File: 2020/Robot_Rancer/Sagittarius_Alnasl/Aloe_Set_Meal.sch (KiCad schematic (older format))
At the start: 235 parts, among them J1 SWD, J10 MOTOR1, J11 MOTOR3, J12 MOTOR5, J13 BATT_IN, J14 3522-2, J15 microSD, J16 SERIAL1, J17 VOLTMETER, J18 TO_VOLTMETER, J2 ADC, J3 ADC_Vdd, J4 SERIAL0, J5 ENC, J6 MOTOR0, J7 MOTOR2, J8 MOTOR4, J9 SERVO, Q1 NVMFD5C446NLT1G, Q10 NVMFD5C446NLT1G, Q11 NVMFD5C446NLT1G, Q12 NVMFD5C446NLT1G, Q13 FET_P, Q14 FET_N, Q15 FET_P, Q16 NPN, Q2 NVMFD5C446NLT1G, Q3 NVMFD5C446NLT1G, Q4 NVMFD5C446NLT1G, Q5 NVMFD5C446NLT1G, Q6 NVMFD5C446NLT1G, Q7 NVMFD5C446NLT1G, Q8 NVMFD5C446NLT1G, Q9 NVMFD5C446NLT1G, SW1 RST, SW2 SW0, SW3 SW1, SW4 EMG, SW5 MAIN_SW, U1 BD9G101G, U10 NCP5104, U11 NCP5104, U12 NCP5104, U13 NCP5104, U14 NCP5104, U15 NCP5104, U16 NCP5104, U17 NCP5104, U18 V23086-C1001, U19 LOGO, U2 MCP2221A, U20 LOGO, U21 LOGO, U22 AQM0802, U23 74HCT04, U24 74HC02, U25 74HC02, U26 74HC02, U27 LOGO, U28 FULLCOLOR, U29 LOGO, U3 STM32F446RETx, U30 LOGO, U4 ROTARY, U5 AZ1086H, U6 NCP5104, U7 NCP5104, U8 NCP5104, U9 NCP5104, Y1 8MHz

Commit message: 抵抗値入れた
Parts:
- removed Q13: FET_P, Package_TO_SOT_SMD:SOT-23W, symbol Device:Q_PMOS_GDS
- removed Q15: FET_P, Package_TO_SOT_SMD:SOT-23W, symbol Device:Q_NMOS_GSD
- added Q13, Q15: FET_P, Package_TO_SOT_SMD:SOT-23, symbol Device:Q_PMOS_GSD
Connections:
- net +5V: now also Q13.3 (D)
- net 5Vc: now also Q13.2 (S)
- net Batt: now also Q15.2 (S)
- net at D27.1 (K), U18.2: now also Q15.3 (D)
- net at R52.2, SW4.2 (B): now also Q15.1 (G)
- net at R65.2, SW5.2 (B): now also Q13.1 (G)
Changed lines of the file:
@@
 Wire Wire Line
 	20700 7950 20750 7950
-Connection ~ 20750 7550
-$Comp
-L Device:Q_PMOS_GDS Q13
-U 1 1 5EA59B7C
-P 20650 7750
-F 0 "Q13" H 20856 7796 50  0000 L CNN
-F 1 "FET_P" H 20856 7705 50  0000 L CNN
-F 2 "Package_TO_SOT_SMD:SOT-23W" H 20850 7850 50  0001 C CNN
-F 3 "~" H 20650 7750 50  0001 C CNN
-	1    20650 7750
-	1    0    0    1
-$EndComp
 Wire Wire Line
 	21625 7550 21625 7725
@@
 Wire Wire Line
 	16350 10850 16325 10850
-$Comp
-L Device:Q_NMOS_GSD Q15
-U 1 1 5EA796FC
-P 3850 1350
-F 0 "Q15" H 4025 1150 50  0000 L CNN
-F 1 "FET_P" H 4025 1225 50  0000 L CNN
-F 2 "Package_TO_SOT_SMD:SOT-23W" H 4050 1450 50  0001 C CNN
-F 3 "~" H 3850 1350 50  0001 C CNN
-	1    3850 1350
-	1    0    0    -1
-$EndComp
 Text GLabel 2875 1200 2    50   Input ~ 0
 5Vc
@@
 Wire Wire Line
 	20600 7025 20750 7025
+$Comp
+L Device:Q_PMOS_GSD Q13
+U 1 1 5E61DA1A
+P 3850 1350
+F 0 "Q13" H 4056 1396 50  0000 L CNN
+F 1 "FET_P" H 4056 1305 50  0000 L CNN
+F 2 "Package_TO_SOT_SMD:SOT-23" H 4050 1450 50  0001 C CNN
+F 3 "~" H 3850 1350 50  0001 C CNN
+	1    3850 1350
+	1    0    0    -1
+$EndComp
+$Comp
+L Device:Q_PMOS_GSD Q15
+U 1 1 5E62C9E6
+P 20650 7750
+F 0 "Q15" H 20856 7796 50  0000 L CNN
+F 1 "FET_P" H 20856 7705 50  0000 L CNN
+F 2 "Package_TO_SOT_SMD:SOT-23" H 20850 7850 50  0001 C CNN
+F 3 "~" H 20650 7750 50  0001 C CNN
+	1    20650 7750
+	1    0    0    -1
+$EndComp
+Connection ~ 20750 7550
 $EndSCHEMATC

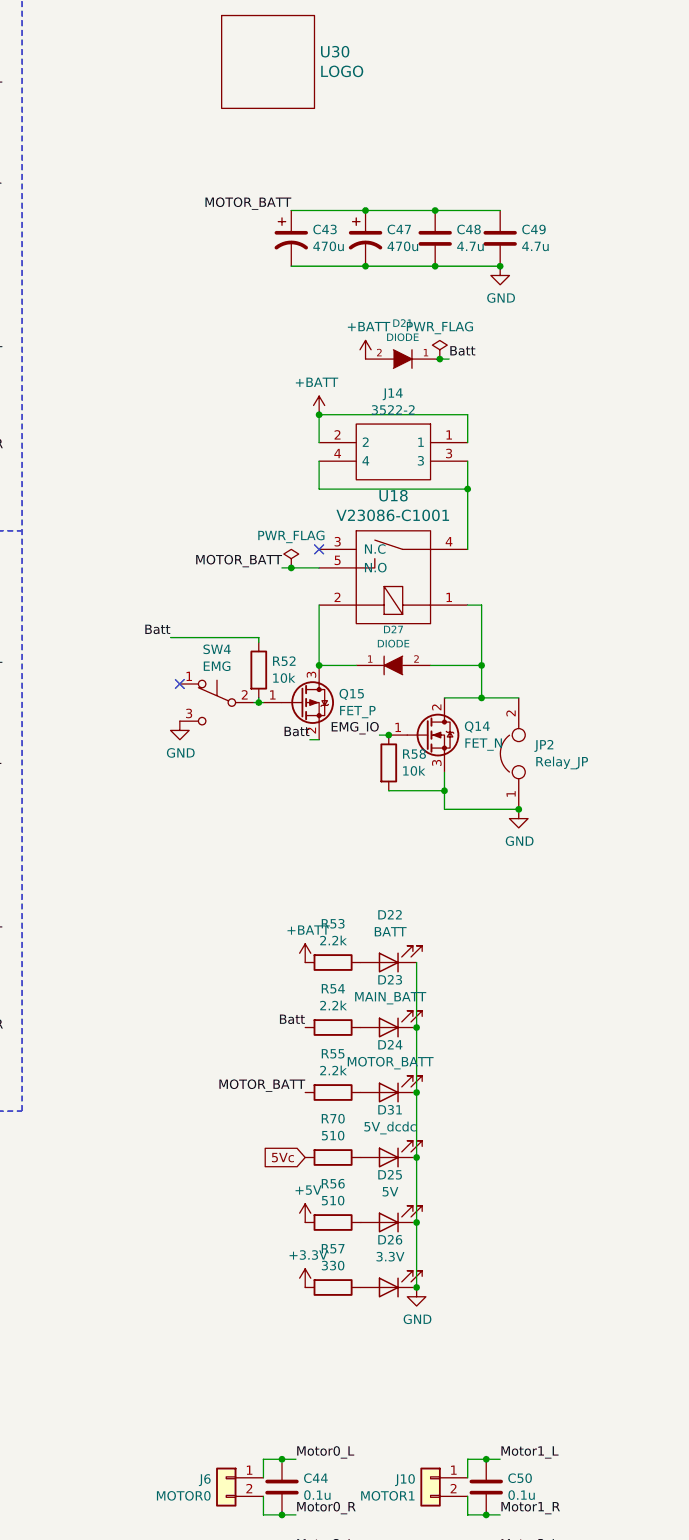
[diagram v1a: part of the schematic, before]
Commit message: 和ランサー基板に機体のロゴを追加した
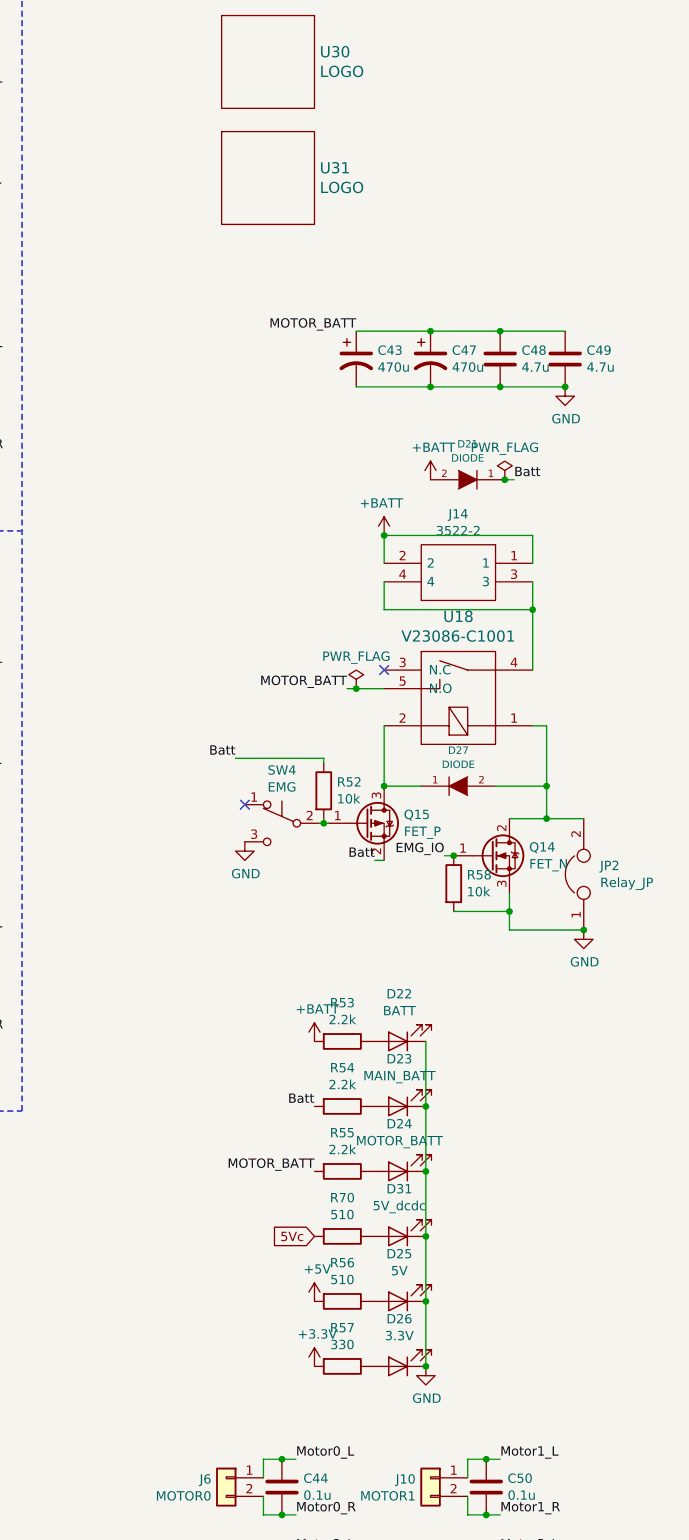
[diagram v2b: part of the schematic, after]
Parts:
- added U31: LOGO, Mizz_lib:kodani_miconCar_30x19_silk, symbol Miz:LOGO
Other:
- moved on the sheet: C43, C47, C48, C49, D21, D22, D23, D24, D25, D26, D27, D31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
